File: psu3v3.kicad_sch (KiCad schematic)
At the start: 26 parts, among them U15 AP64501SP-13

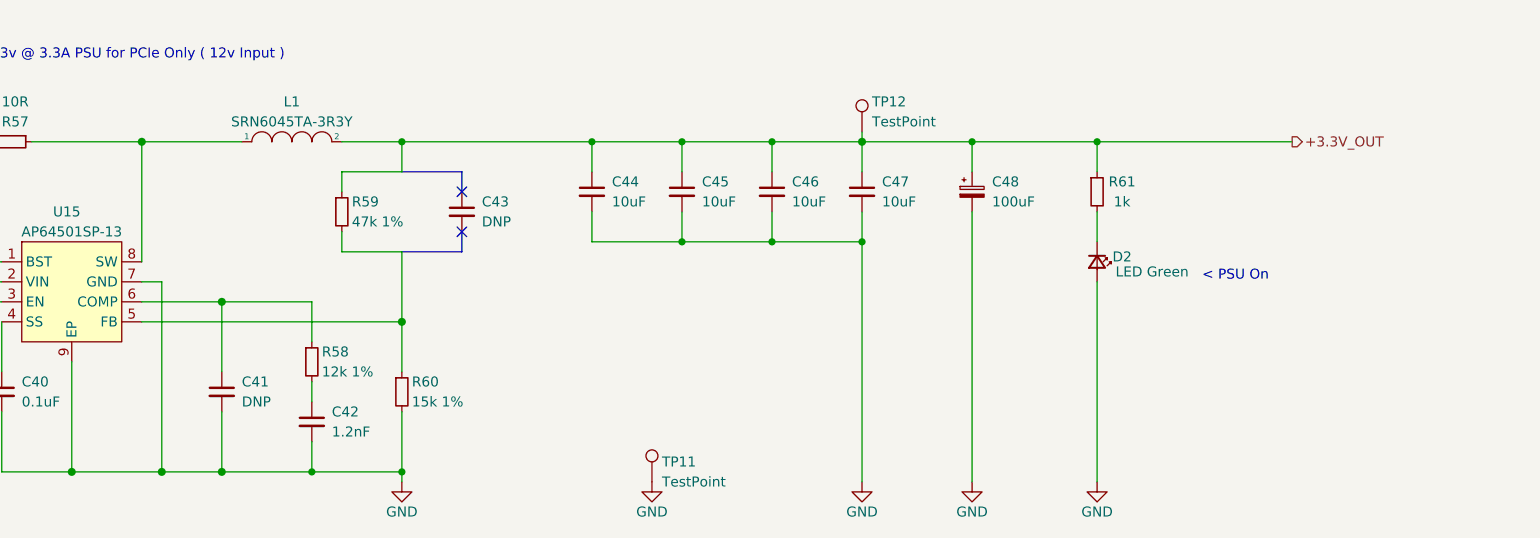
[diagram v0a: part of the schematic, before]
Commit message: leds
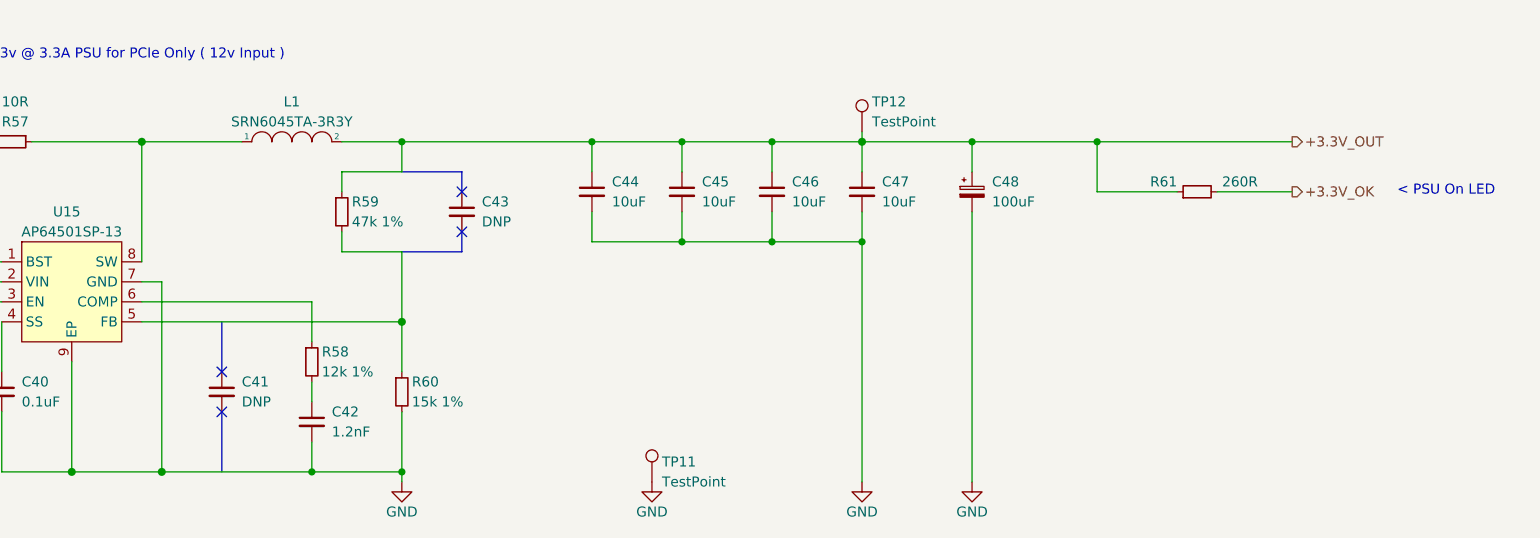
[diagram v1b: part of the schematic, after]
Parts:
- removed D2: LED Green, LED_SMD_LiteOn:LED_0603_1608Metric_green, symbol LED_SMD_LiteOn:LED Green
- C41: now left out of the parts list
- R61: value 1k -> 260R
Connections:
- net GND: no longer C41.2
- net +3.3V_OK: now reaches R61.2
- net at R58.1, U15.6 (COMP): no longer C41.1
- no-connect marks 2 -> 4
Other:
- note added: "< PSU On LED"
- note removed: "< PSU On"
- moved on the sheet: R61
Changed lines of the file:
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@@
   (junction (at 106.68 156.21) (diameter 0.9144) (color 0 0 0 0)
   )
-  (junction (at 196.85 170.18) (diameter 1.016) (color 0 0 0 0)
-  )
   (junction (at 266.7 140.97) (diameter 0.9144) (color 0 0 0 0)
   )
@@
   )
   (junction (at 91.44 156.21) (diameter 0.9144) (color 0 0 0 0)
-  )
-  (junction (at 196.85 148.59) (diameter 1.016) (color 0 0 0 0)
   )
   (no_connect (at 227.33 139.7))
   (no_connect (at 227.33 134.62))
+  (no_connect (at 196.85 162.56))
+  (no_connect (at 196.85 157.48))
   (wire (pts (xy 212.09 132.08) (xy 212.09 134.62))
     (stroke (width 0) (type solid) (color 0 0 0 0))
@@
     (stroke (width 0) (type solid) (color 0 0 0 0))
   )
+  (wire (pts (xy 323.215 134.62) (xy 332.74 134.62))
+    (stroke (width 0) (type default) (color 0 0 0 0))
+  )
   (wire (pts (xy 243.84 132.08) (xy 243.84 128.27))
-    (stroke (width 0) (type solid) (color 0 0 0 0))
-  )
-  (wire (pts (xy 196.85 148.59) (xy 196.85 157.48))
     (stroke (width 0) (type solid) (color 0 0 0 0))
   )
@@
     (stroke (width 0) (type solid) (color 0 0 0 0))
   )
-  (wire (pts (xy 196.85 162.56) (xy 196.85 170.18))
-    (stroke (width 0) (type solid) (color 0 0 0 0))
-  )
-  (wire (pts (xy 186.69 148.59) (xy 196.85 148.59))
+  (wire (pts (xy 186.69 148.59) (xy 208.28 148.59))
     (stroke (width 0) (type solid) (color 0 0 0 0))
   )
@@
     (stroke (width 0) (type solid) (color 0 0 0 0))
   )
+  (polyline (pts (xy 196.85 151.13) (xy 196.85 157.48))
+    (stroke (width 0) (type default) (color 0 0 0 0))
+  )
   (wire (pts (xy 158.75 143.51) (xy 168.91 143.51))
     (stroke (width 0) (type solid) (color 0 0 0 0))
@@
     (stroke (width 0) (type solid) (color 0 0 0 0))
   )
-  (wire (pts (xy 307.975 128.27) (xy 307.975 132.08))
+  (wire (pts (xy 307.975 128.27) (xy 307.975 134.62))
     (stroke (width 0) (type solid) (color 0 0 0 0))
   )
@@
   )
   (wire (pts (xy 212.09 132.08) (xy 219.71 132.08))
-    (stroke (width 0) (type solid) (color 0 0 0 0))
-  )
-  (wire (pts (xy 196.85 148.59) (xy 208.28 148.59))
     (stroke (width 0) (type solid) (color 0 0 0 0))
   )
@@
     (stroke (width 0) (type default) (color 0 0 0 0))
   )
-  (wire (pts (xy 307.975 137.16) (xy 307.975 140.97))
-    (stroke (width 0) (type solid) (color 0 0 0 0))
-  )
   (wire (pts (xy 212.09 139.7) (xy 212.09 142.24))
     (stroke (width 0) (type solid) (color 0 0 0 0))
   )
-  (wire (pts (xy 196.85 170.18) (xy 208.28 170.18))
-    (stroke (width 0) (type solid) (color 0 0 0 0))
-  )
   (wire (pts (xy 208.28 170.18) (xy 219.71 170.18))
     (stroke (width 0) (type solid) (color 0 0 0 0))
@@
     (stroke (width 0) (type solid) (color 0 0 0 0))
   )
-  (wire (pts (xy 189.23 170.18) (xy 196.85 170.18))
+  (wire (pts (xy 189.23 170.18) (xy 208.28 170.18))
     (stroke (width 0) (type solid) (color 0 0 0 0))
   )
@@
   (wire (pts (xy 255.27 132.08) (xy 255.27 128.27))
     (stroke (width 0) (type solid) (color 0 0 0 0))
+  )
+  (polyline (pts (xy 196.85 162.56) (xy 196.85 170.18))
+    (stroke (width 0) (type default) (color 0 0 0 0))
   )
   (wire (pts (xy 177.8 170.18) (xy 189.23 170.18))
@@
     (stroke (width 0) (type solid) (color 0 0 0 0))
   )
+  (wire (pts (xy 307.975 134.62) (xy 318.135 134.62))
+    (stroke (width 0) (type default) (color 0 0 0 0))
+  )
   (wire (pts (xy 186.69 151.13) (xy 219.71 151.13))
     (stroke (width 0) (type solid) (color 0 0 0 0))
@@
   )
   (wire (pts (xy 212.09 128.27) (xy 219.71 128.27))
-    (stroke (width 0) (type solid) (color 0 0 0 0))
-  )
-  (wire (pts (xy 307.975 146.05) (xy 307.975 171.45))
     (stroke (width 0) (type solid) (color 0 0 0 0))
   )
@@
     (effects (font (size 5 5) (thickness 1) bold italic) (justify left bottom))
   )
-  (text "< PSU On" (at 321.31 146.05 0)
+  (text "< PSU On LED" (at 346.075 135.255 0)
     (effects (font (size 1.27 1.27)) (justify left bottom))
   )
@@
     (effects (font (size 1.27 1.27)) (justify right))
   )
+  (hierarchical_label "+3.3V_OK" (shape output) (at 332.74 134.62 0)
+    (effects (font (size 1.27 1.27)) (justify left))
+  )
   (symbol (lib_id "Device:C_Small") (at 168.91 160.02 0) (unit 1)
     (in_bom yes) (on_board yes)
@@
     )
     (property "Part Description" "10uF 10% 10V Ceramic Capacitor X7R 0805 (2012 Metric)" (id 8) (at 278.13 134.62 0)
-      (effects (font (size 1.27 1.27)) hide)
-    )
-    (pin "1")
-    (pin "2")
-  )
-  (symbol (lib_id "LED_SMD_LiteOn:LED Green") (at 307.975 143.51 270) (unit 1)
-    (in_bom yes) (on_board yes)
-    (property "Reference" "D2" (id 0) (at 311.15 142.875 90))
-    (property "Value" "LED Green" (id 1) (at 314.96 144.78 90))
-    (property "Footprint" "LED_SMD_LiteOn:LED_0603_1608Metric_green" (id 2) (at 297.815 143.51 0)
-      (effects (font (size 1.27 1.27)) hide)
-    )
-    (property "Datasheet" "" (id 3) (at 307.975 143.51 90)
-      (effects (font (size 1.27 1.27)) hide)
-    )
-    (property "Manufacturer" "Lite-On" (id 4) (at 302.895 143.51 0)
-      (effects (font (size 1.27 1.27)) hide)
-    )
-    (property "MPN" "LTST-C193KGKT-5A" (id 5) (at 300.355 143.51 0)
       (effects (font (size 1.27 1.27)) hide)
     )
@@
     (pin "1")
   )
-  (symbol (lib_id "Device:R_Small") (at 307.975 134.62 0) (unit 1)
-    (in_bom yes) (on_board yes)
-    (property "Reference" "R61" (id 0) (at 311.15 133.35 0))
-    (property "Value" "1k" (id 1) (at 311.15 135.89 0))
-    (property "Footprint" "Resistor_SMD:R_0402_1005Metric" (id 2) (at 307.975 134.62 0)
-      (effects (font (size 1.27 1.27)) hide)
-    )
-    (property "Datasheet" "~" (id 3) (at 307.975 134.62 0)
+  (symbol (lib_id "Device:R_Small") (at 320.675 134.62 90) (unit 1)
+    (in_bom yes) (on_board yes)
+    (property "Reference" "R61" (id 0) (at 318.135 133.35 90)
+      (effects (font (size 1.27 1.27)) (justify left))
+    )
+    (property "Value" "260R" (id 1) (at 323.85 133.35 90)
+      (effects (font (size 1.27 1.27)) (justify right))
+    )
+    (property "Footprint" "Resistor_SMD:R_0402_1005Metric" (id 2) (at 320.675 134.62 0)
+      (effects (font (size 1.27 1.27)) hide)
+    )
+    (property "Datasheet" "~" (id 3) (at 320.675 134.62 0)
       (effects (font (size 1.27 1.27)) hide)
     )
@@
     (pin "1")
     (pin "2")
-  )
-  (symbol (lib_id "power:GND") (at 307.975 171.45 0) (unit 1)
-    (in_bom yes) (on_board yes)
-    (property "Reference" "#PWR048" (id 0) (at 307.975 177.8 0)
-      (effects (font (size 1.27 1.27)) hide)
-    )
-    (property "Value" "GND" (id 1) (at 307.975 175.26 0))
-    (property "Footprint" "" (id 2) (at 307.975 171.45 0)
-      (effects (font (size 1.27 1.27)) hide)
-    )
-    (property "Datasheet" "" (id 3) (at 307.975 171.45 0)
-      (effects (font (size 1.27 1.27)) hide)
-    )
-    (pin "1")
   )
   (symbol (lib_id "Device:C_Small") (at 266.7 134.62 0) (unit 1)
@@
   )
   (symbol (lib_id "Device:C_Small") (at 196.85 160.02 0) (unit 1)
-    (in_bom yes) (on_board yes)
+    (in_bom no) (on_board no)
     (property "Reference" "C41" (id 0) (at 199.39 158.75 0)
       (effects (font (size 1.27 1.27)) (justify left))
